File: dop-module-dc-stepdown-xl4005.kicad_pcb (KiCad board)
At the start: 4 copper layers, 50.8 x 38.1 mm, 16 parts, among them J101 Input, J102 Output, U101 XL4005

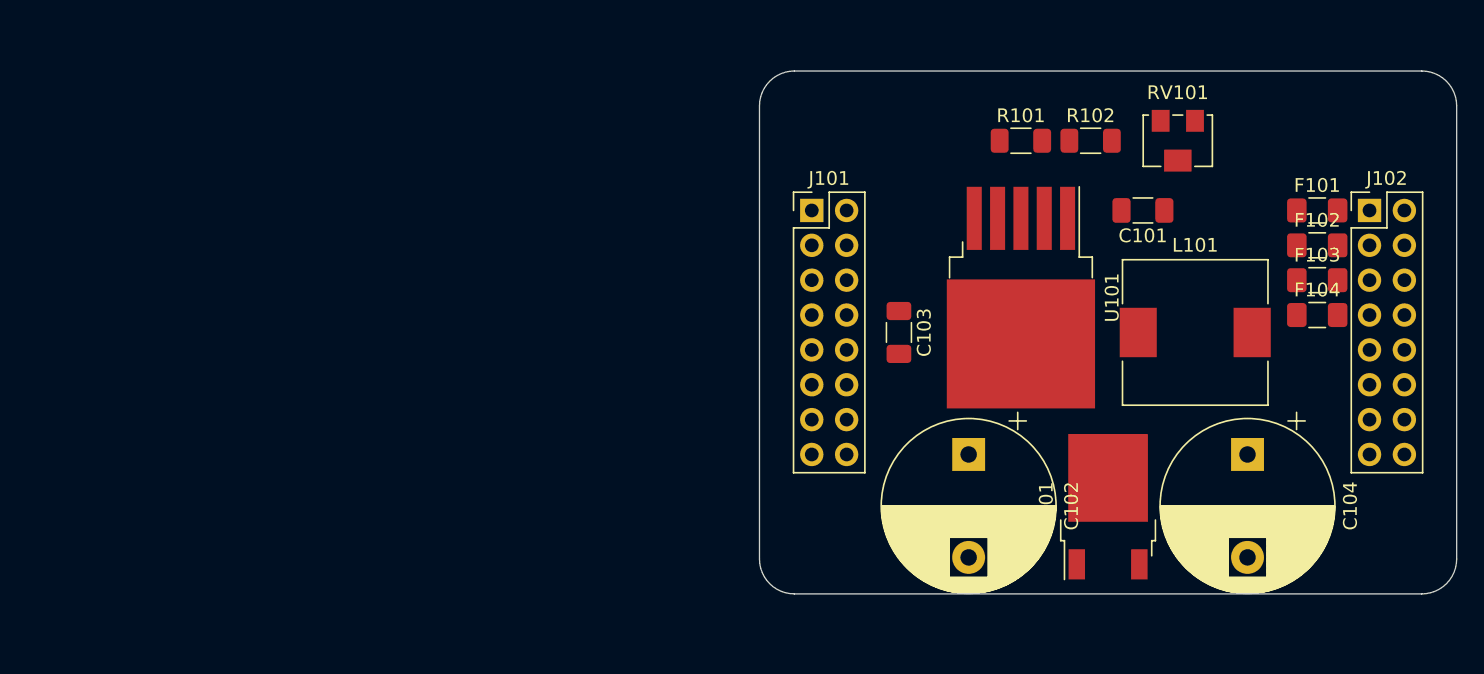
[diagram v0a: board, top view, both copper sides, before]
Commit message: complete rework
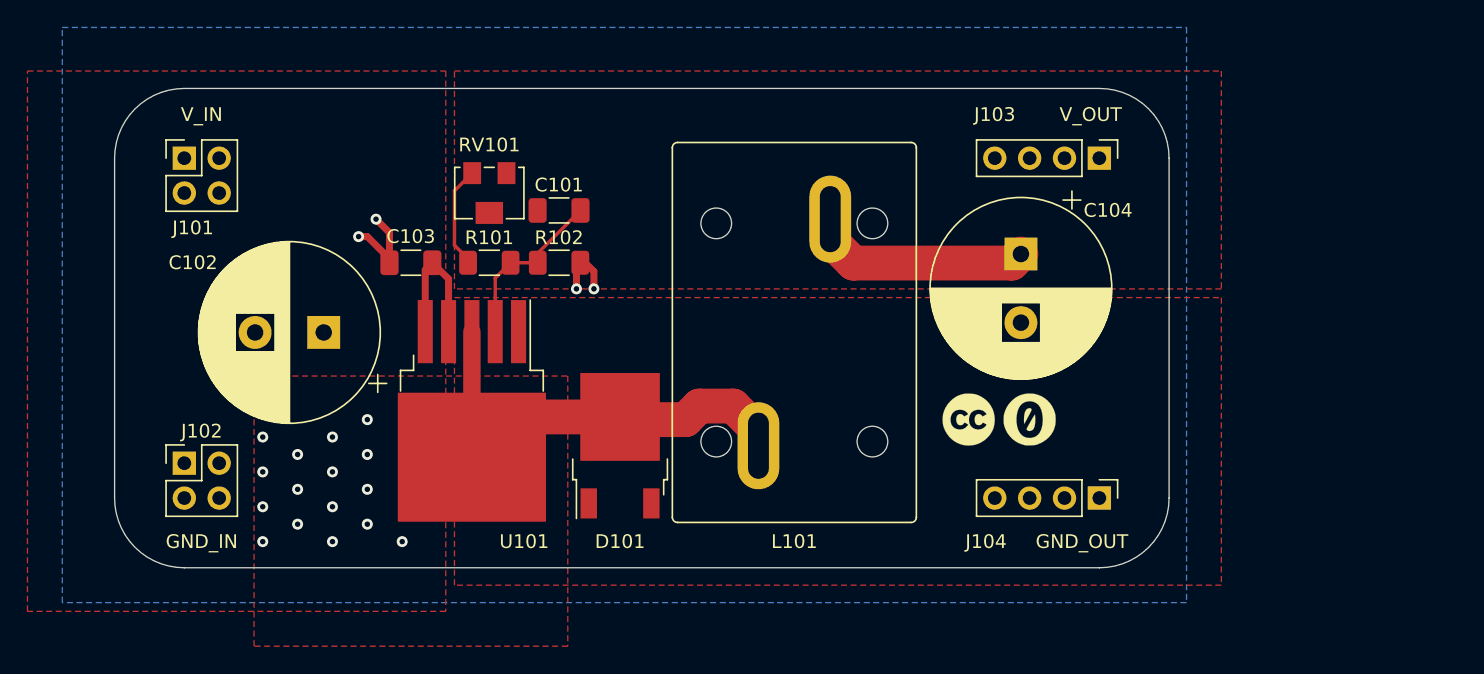
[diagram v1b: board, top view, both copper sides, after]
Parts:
- removed F101, F102, F103, F104: 1A, Fuse:Fuse_1206_3216Metric_Pad1.42x1.75mm_HandSolder
- added G***: LOGO, cliparts:logo--cc--zero, F.Cu at (95.9, 177.8)
- added G***: LOGO, cliparts:logo--cc--cc, F.Cu at (91.4, 177.8)
- added J103: V_OUT, Connector_PinHeader_2.54mm:PinHeader_1x04_P2.54mm_Vertical, F.Cu at (101.0, 158.8)
- added J104: GND_OUT, Connector_PinHeader_2.54mm:PinHeader_1x04_P2.54mm_Vertical, F.Cu at (101.0, 183.5)
- C102, C104: footprint Capacitor_THT:CP_Radial_D12.5mm_P7.50mm -> Capacitor_THT:CP_Radial_D13.0mm_P5.00mm
- J101: value Input -> V_IN; footprint Connector_PinHeader_2.54mm:PinHeader_2x08_P2.54mm_Vertical -> Connector_PinHeader_2.54mm:PinHeader_2x02_P2.54mm_Vertical
- J102: value Output -> GND_IN; footprint Connector_PinHeader_2.54mm:PinHeader_2x08_P2.54mm_Vertical -> Connector_PinHeader_2.54mm:PinHeader_2x02_P2.54mm_Vertical
- L101: footprint Inductor_SMD:L_10.4x10.4_H4.8 -> coilcraft_THT:CoilCraft_AGP2923
- moved J102 88.3 mm to (34.3, 181.0)
- moved RV101 50.3 mm to (56.5, 161.3)
- moved C102 47.8 mm to (44.5, 171.4), turned to 180 degrees
- moved J101 45.9 mm to (34.3, 158.8)
- moved C101 42.5 mm to (61.6, 162.6), turned to 0 degrees
- moved U101 40.8 mm to (55.2, 177.2)
- moved R101 39.7 mm to (56.5, 166.4)
- moved R102 39.7 mm to (61.6, 166.4)
- moved C103 35.9 mm to (50.8, 166.4), turned to 180 degrees
- moved D101 35.8 mm to (66.0, 179.7)
- moved L101 29.2 mm to (78.7, 171.4), turned to 90 degrees
- moved C104 22.0 mm to (95.2, 165.7)
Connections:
- J102 pad 1: Net-(F101-Pad1) -> GND
- J102 pad 2: Net-(F101-Pad1) -> GND
- J102 pad 3: Net-(F101-Pad1) -> GND
- J102 pad 4: Net-(F101-Pad1) -> GND
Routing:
- net Net-(D101-Pad2): track 0.00 -> 33.6 mm, vias 0 -> 16
- net +5V: track 0.00 -> 16.4 mm
- net Net-(C101-Pad2): track 0.00 -> 12.6 mm
- net GND: track 0.00 -> 11.3 mm, vias 0 -> 4
- net +15V: track 0.00 -> 10.7 mm
- net Net-(R101-Pad1): track 0.00 -> 7.47 mm
- added copper zone on F.Cu, net +15V
- added copper zone on F.Cu, net +5V
- added copper zone on B.Cu, net GND
- added copper zone on F.Cu, net GND
- added copper zone on F.Cu, net Net-(D101-Pad2)
- removed copper zone on In1.Cu, net GND
- removed copper zone on In2.Cu, net GND
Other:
- board size 50.8 x 38.1 mm -> 76.8 x 34.9 mm
